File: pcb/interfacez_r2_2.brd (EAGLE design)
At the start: 100 x 50 mm, 171 parts, among them IC1 STMPS2141STR, IC10 74LCX245FT, IC11 74LCX245FT, IC12 USB1T11AMTCX, IC2 EP4CE6E22C8N, IC3 74LCX245FT, IC4 74LCX245FT, IC5 MP2233DJ, IC6 MP2233DJ, IC7 CH330N, IC8 MIC5504-2.5YM5-TR, IC9 LY68L6400SLIT, J1 AMPHENOL_ICC_-_FCI_20021121-0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, Q1 BSS123, Q2 BSS123, Q3 CJ3439KDW, Q4 CJ3439KDW, Q5 BSS84, Q6 BSS123, U1 ESP-WROOM-32

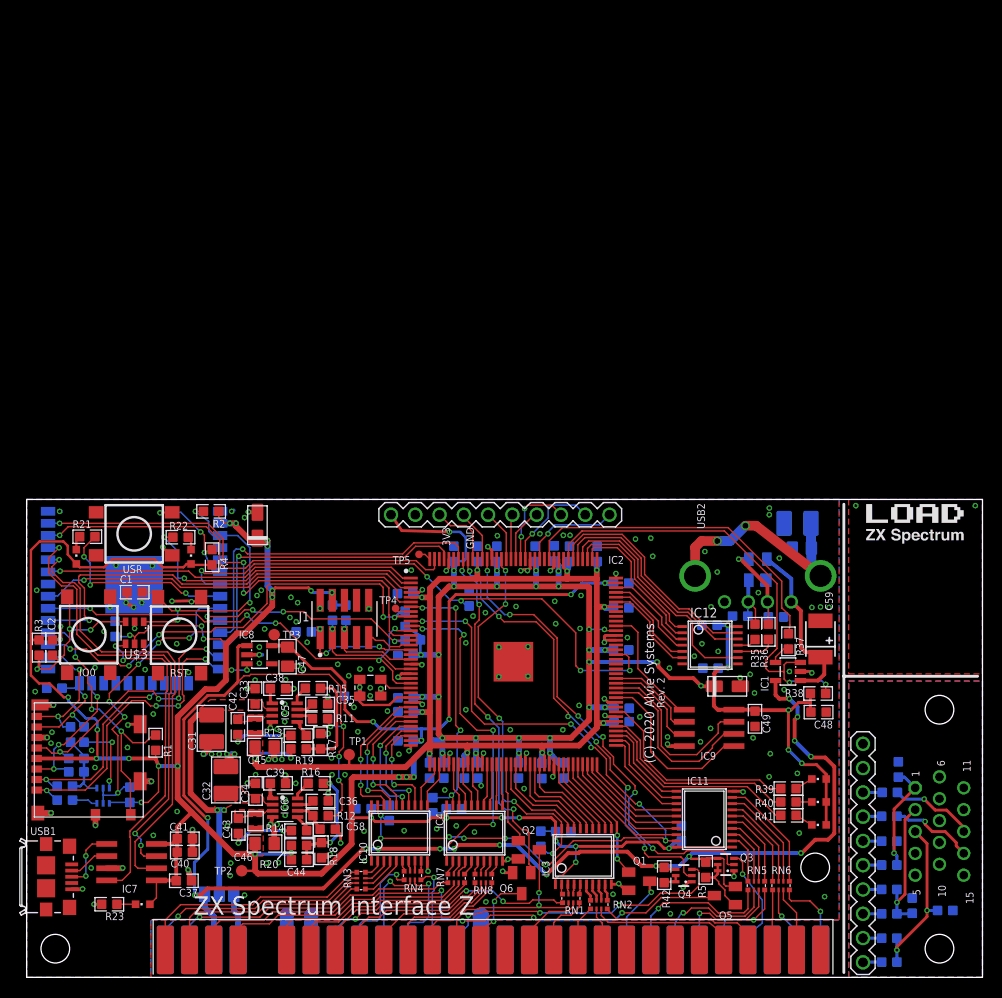
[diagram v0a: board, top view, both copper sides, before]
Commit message: New board layout
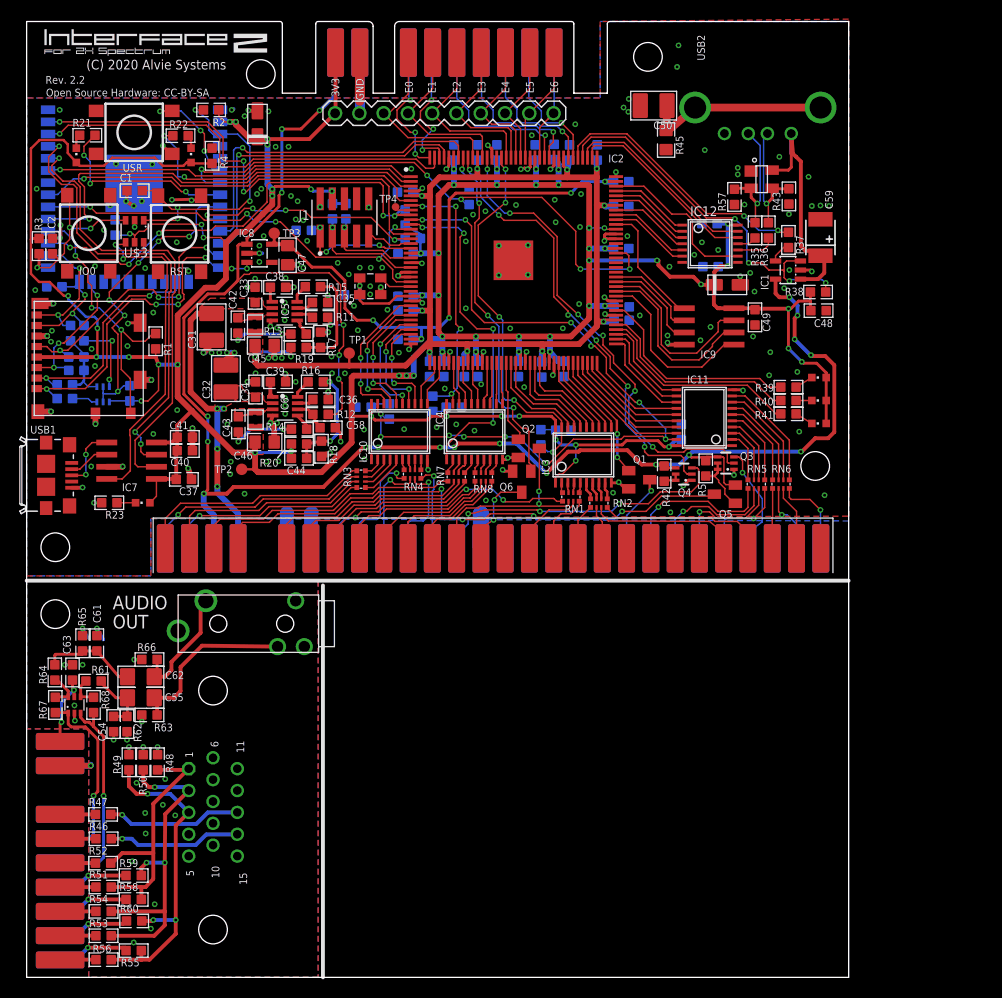
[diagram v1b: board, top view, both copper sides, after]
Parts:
- removed SJ1: (no value), jumper:SJ_2
- removed TP5: TPTP08R, testpad:TP08R
- removed U$2: PIN-1X10, alvie:PIN-1X10
- added C54, C61, C63: 100nF, GadgetFactory:0603
- added C55, C62: 47uF, GadgetFactory:1206
- added IC13: NC7WZ16P6X, GadgetFactory:SC70-6
- added R58: 520R, GadgetFactory:0603
- added R59, R60: 270R, GadgetFactory:0603
- added R61, R64: 220R, GadgetFactory:0603
- added R62, R65: 100R, GadgetFactory:0603
- added R63, R66: 1K8, GadgetFactory:0603
- added R67, R68: 0R/DNP, GadgetFactory:0603
- added U$5, U$8: INTERFACEZ_EDGEDAUGHTER, alvie:INTERFACEZ_EXPANSION_DAUGHTERCARD
- added U$9: PJ328-A0, alvie:PJ328A0
- moved R50 86.8 mm to (10.7, 22.5), flipped to the top, turned to 270 degrees
- moved R47 82.3 mm to (8.00, 17.1), flipped to the top, turned to 0 degrees
- moved R52 82.3 mm to (8.00, 11.9), flipped to the top, turned to 0 degrees
- moved R46 82.2 mm to (8.05, 14.5), flipped to the top, turned to 0 degrees
- moved R51 82.2 mm to (8.05, 9.45), flipped to the top, turned to 0 degrees
- moved R53 82.2 mm to (8.05, 4.35), flipped to the top, turned to 0 degrees
- moved R54 82.2 mm to (8.05, 6.90), flipped to the top, turned to 0 degrees
- moved R56 82.2 mm to (8.05, 1.85), flipped to the top, turned to 0 degrees
- moved R49 81.8 mm to (12.2, 22.5), flipped to the top
- moved R55 79.1 mm to (11.2, 2.80), flipped to the top, turned to 0 degrees
- moved R48 77.5 mm to (13.7, 22.5), flipped to the top
- moved X1 76.0 mm to (19.5, 17.5)
- moved USB2 49.0 mm to (76.5, 91.0)
- moved C50 46.2 mm to (65.6, 91.2), flipped to the top, turned to 180 degrees
- moved R45 45.0 mm to (66.9, 87.6), flipped to the top, turned to 270 degrees
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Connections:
- removed net N$66: J1.7
- removed net N$70: J1.6
- removed net N$71: J1.8
- removed net SPEED: IC12.9, IC2.112
- removed net VREG: C31.2, C32.2, C33.2, C34.2, IC5.2, IC6.2, SJ1.2
- new net AUDIO_L: IC13.3, R68.1, U$8.A6
- new net AUDIO_R: IC13.1, R67.1, U$8.A5
- new net BLUE2: R60.1, U$8.A9
- new net BUF_L: IC13.6, R64.2, R67.2
- new net BUF_R: IC13.4, R61.2, R68.2
- new net EXT10: IC2.115, U$5.A8
- new net EXT11: IC2.114, U$5.A9
- new net EXT12: IC2.142, U$5.A5
- new net EXT13: IC2.144, U$5.A4
- new net EXT8: IC2.120, U$5.A6
- new net EXT9: IC2.119, U$5.A7
- new net GREEN2: R59.1, U$8.A7
- new net LL: C62.2, R66.1, U$9.2
- new net LR: C55.2, R63.1, U$9.3
- new net N$67: C61.2, C62.1, R64.1, R65.1
- new net N$68: C54.2, C55.1, R61.1, R62.1
- new net RED2: R58.1, U$8.A8
- new net USB_SPEED: IC12.9, IC2.106
- net +3V3: now also C63.2, IC13.5, U$5.B1, U$8.B1; no longer U$2.1
- net +5V: now also U$5.A1; no longer SJ1.1
- net +9V: now also C31.2, C32.2, C33.2, C34.2, IC5.2, IC6.2; no longer SJ1.3
- net BLUE: now also R60.2
- net BLUE0: now also U$8.A10; no longer U$2.10
- net BLUE1: now also U$8.B10; no longer U$2.9
- net EXT0: now also U$5.B4
- net EXT1: now also U$5.B5
- net EXT2: now also U$5.B6
- net EXT3: now also U$5.B7
- net EXT4: now also U$5.B8
- net EXT5: now also U$5.B9
- net EXT6: now also U$5.B10
- net EXT7: now also U$5.A10
- net GND: now also C54.1, C61.1, C63.1, IC13.2, R62.2, R63.2, R65.2, R66.2, U$5.A2, U$5.B2, U$8.A2, U$8.B2, U$9.1; no longer U$2.2
- net GREEN: now also R59.2
- net GREEN0: now also U$8.B9; no longer U$2.8
- net GREEN1: now also U$8.B8; no longer U$2.7
- net HSYNC: now also U$8.B4; no longer U$2.3
- net N$55: now also U$8.A1; no longer IC2.144, TP5.TP
- net RCV: now also IC2.103; no longer IC2.106
- net RED: now also R58.2
- net RED0: now also U$8.B7; no longer U$2.6
- net RED1: now also U$8.B6; no longer U$2.5
- net USB_FLT: now also IC2.112; no longer IC2.115
- net USB_MODE: now also IC2.105; no longer IC2.111
- net USB_OE: now also IC2.104; no longer IC2.110
- net USB_PWREN: now also IC2.113; no longer IC2.119
- net USB_SUSPEND: now also IC2.99; no longer IC2.103
- net VM: now also IC2.100; no longer IC2.104
- net VMO: now also IC2.111; no longer IC2.114
- net VP: now also IC2.101; no longer IC2.105
- net VPO: now also IC2.110; no longer IC2.113
- net VSYNC: now also U$8.B5; no longer U$2.4
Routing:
- net GND: track 112.0 -> 163.4 mm, vias 206 -> 231
- net +3V3: track 484.5 -> 529.0 mm, vias 69 -> 70
- net SPEED: track 25.4 -> 0.00 mm
- net +9V: track 6.01 -> 29.8 mm, vias 0 -> 4
- net VREG: track 23.1 -> 0.00 mm, vias 2 -> 0
- net +5V: track 172.7 -> 195.4 mm, vias 19 -> 23
- net AUDIO_L: track 0.00 -> 22.6 mm, vias 0 -> 1
- net GREEN: track 14.7 -> 36.6 mm, vias 1 -> 3
- net AUDIO_R: track 0.00 -> 20.1 mm, vias 0 -> 1
- net EXT8: track 0.00 -> 18.7 mm, vias 0 -> 1
- net LR: track 0.00 -> 18.5 mm
- net USB_SPEED: track 0.00 -> 17.3 mm
- net EXT9: track 0.00 -> 17.2 mm, vias 0 -> 1
- net BLUE: track 17.8 -> 34.8 mm, vias 2 -> 3
- net EXT10: track 0.00 -> 15.7 mm, vias 0 -> 1
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- added copper zone on layer 1, net +9V
- removed copper zone on layer 1, net VREG
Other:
- board size 100 x 50 mm -> 86 x 100 mm
- board text added: "AUDIO"
- board text added: "E0"
- board text added: "E1"
- board text added: "E10"
- board text added: "E11"
- board text added: "E12"
- board text added: "E13"
- board text added: "E2"
- board text added: "E3"
- board text added: "E4"
- board text added: "E5"
- board text added: "E6"
- board text added: "E7"
- board text added: "E8"
- board text added: "E9"
- board text added: "OUT"
- board text added: "Open Source Hardware: CC-BY-SA"
- board text added: "Rev. 2.2"
- board text removed: "+9V"
- board text removed: "Rev. 2"
- board text removed: "ZX Spectrum Interface Z"
